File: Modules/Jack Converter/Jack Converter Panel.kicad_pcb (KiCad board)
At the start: 2 copper layers, 50 x 200 mm, 38 parts

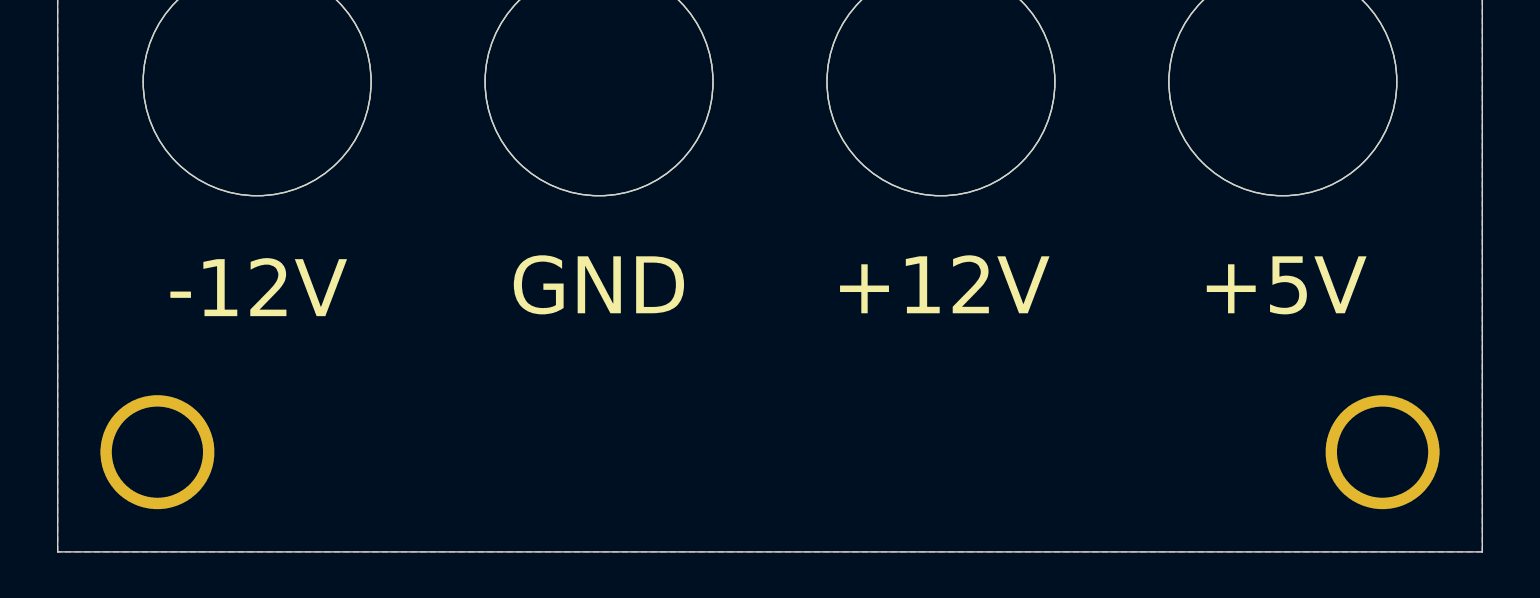
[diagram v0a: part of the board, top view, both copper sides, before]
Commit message: Finished
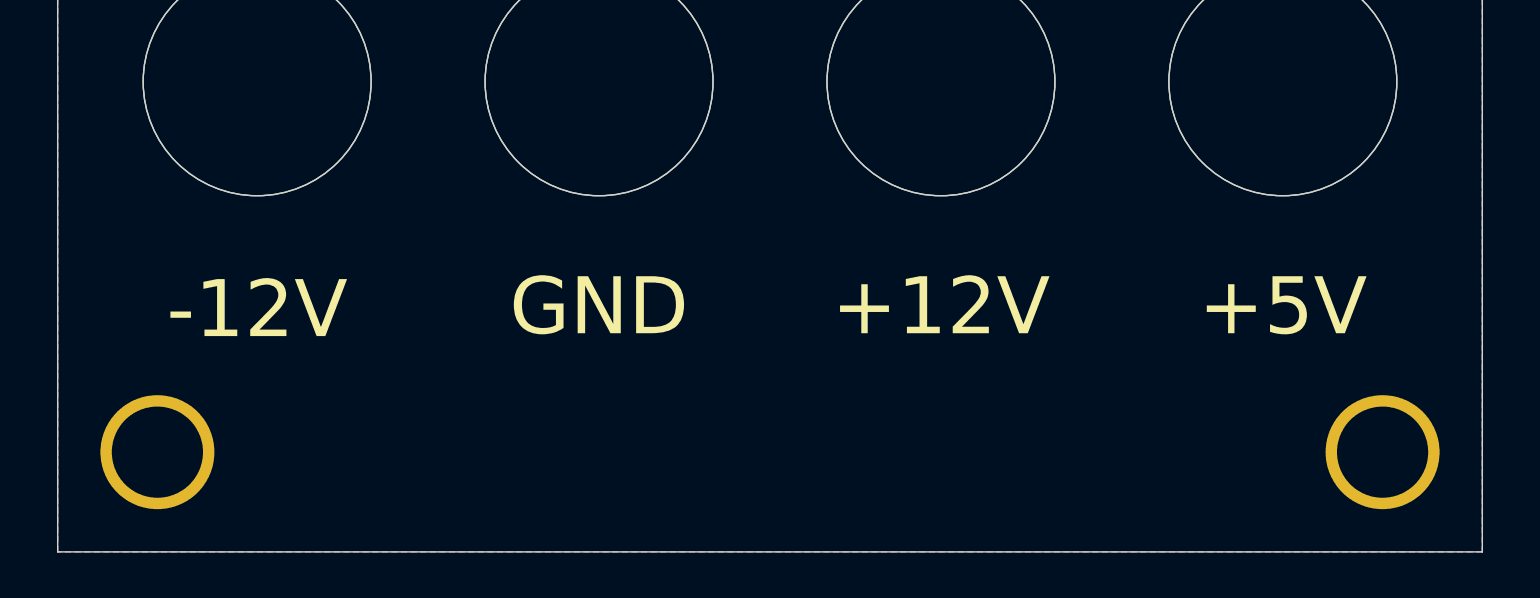
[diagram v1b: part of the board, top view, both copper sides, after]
